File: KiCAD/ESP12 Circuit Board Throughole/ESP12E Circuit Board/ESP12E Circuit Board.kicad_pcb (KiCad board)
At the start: 2 copper layers, 13 parts, among them J1 Conn_01x04_Male, J2 Conn_01x02_Female, Q1 BD437, Q2 BD437, Q3 BD437, U1 ESP8266-12E_ESP-12E, U2 SPX3819M5-L-3-3

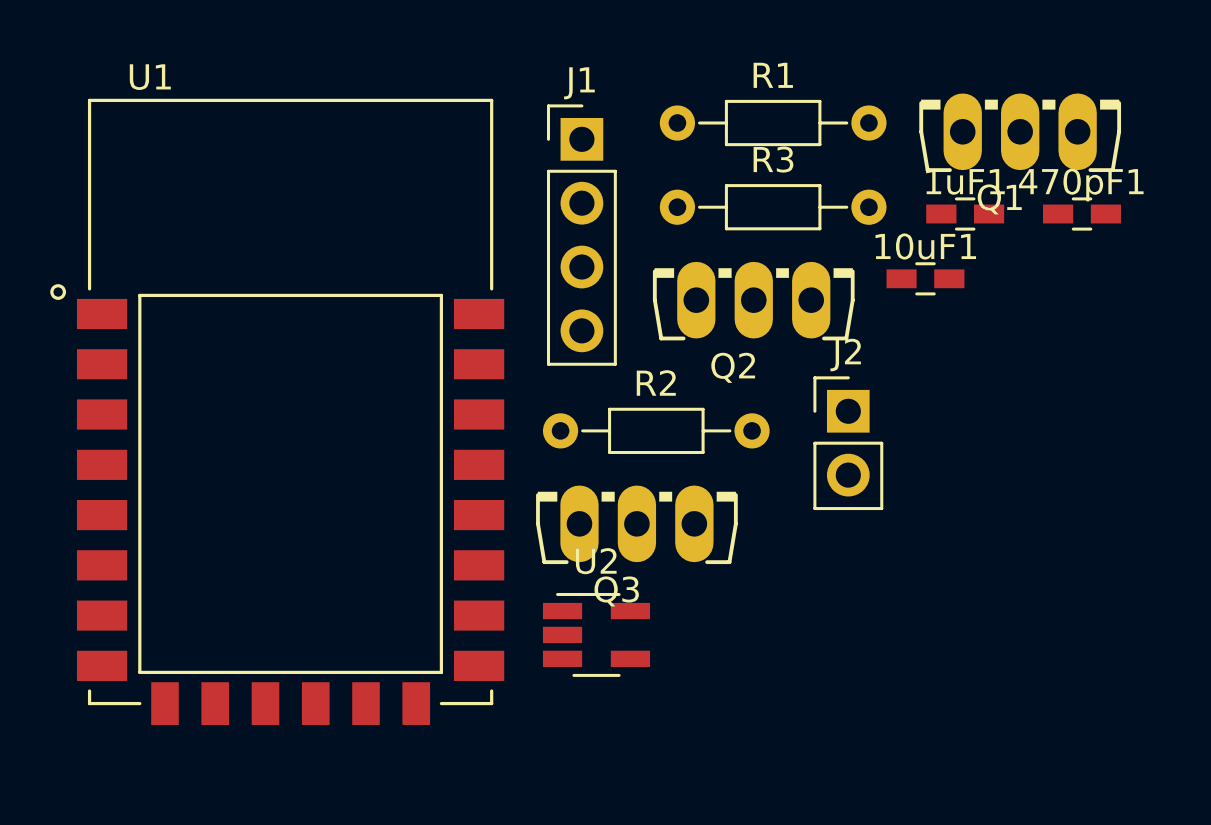
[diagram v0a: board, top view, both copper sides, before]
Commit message: worked on tht circuit
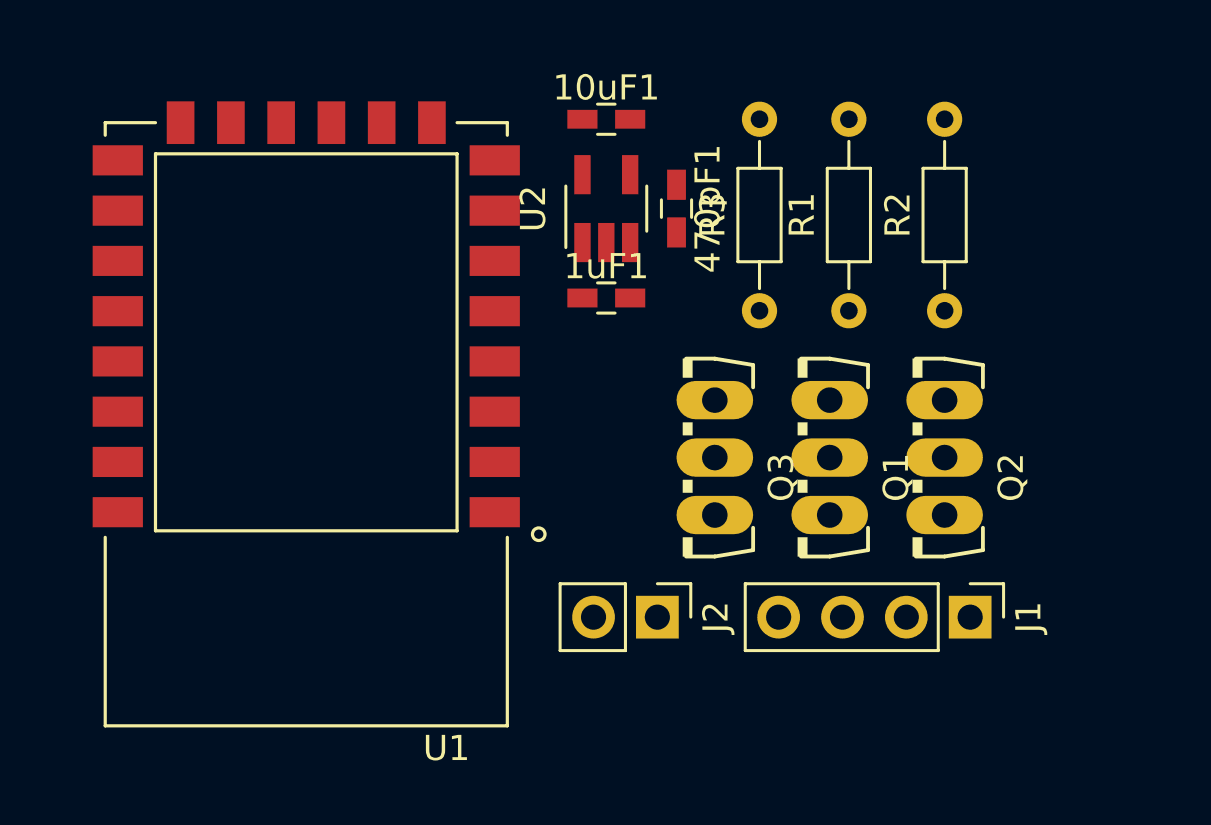
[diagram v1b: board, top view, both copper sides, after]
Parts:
- moved J1 24.5 mm to (161.3, 108.7), turned to 270 degrees
- moved U2 17.0 mm to (146.8, 92.5), turned to 90 degrees
- moved Q1 16.8 mm to (154.4, 102.4), turned to 90 degrees
- moved 470pF1 16.1 mm to (149.6, 92.5), turned to 270 degrees
- moved R2 16.0 mm to (160.3, 96.5), turned to 90 degrees
- moved 1uF1 14.7 mm to (146.8, 96.0)
- moved 10uF1 14.2 mm to (146.8, 88.9)
- moved J2 11.2 mm to (148.8, 108.7), turned to 270 degrees
- moved R1 10.1 mm to (156.5, 96.5), turned to 90 degrees
- moved Q2 9.84 mm to (159.0, 102.4), turned to 90 degrees
- moved U1 6.15 mm to (134.9, 97.5), turned to 180 degrees
- moved R3 5.26 mm to (152.9, 96.5), turned to 90 degrees
- moved Q3 2.28 mm to (149.9, 102.4), turned to 90 degrees
